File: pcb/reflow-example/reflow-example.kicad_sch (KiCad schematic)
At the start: 24 parts, among them U1 NE555D, U2 74LS47, U3 KCSA02-105, U4 74LS393, U5 74LS47, U6 KCSA02-105

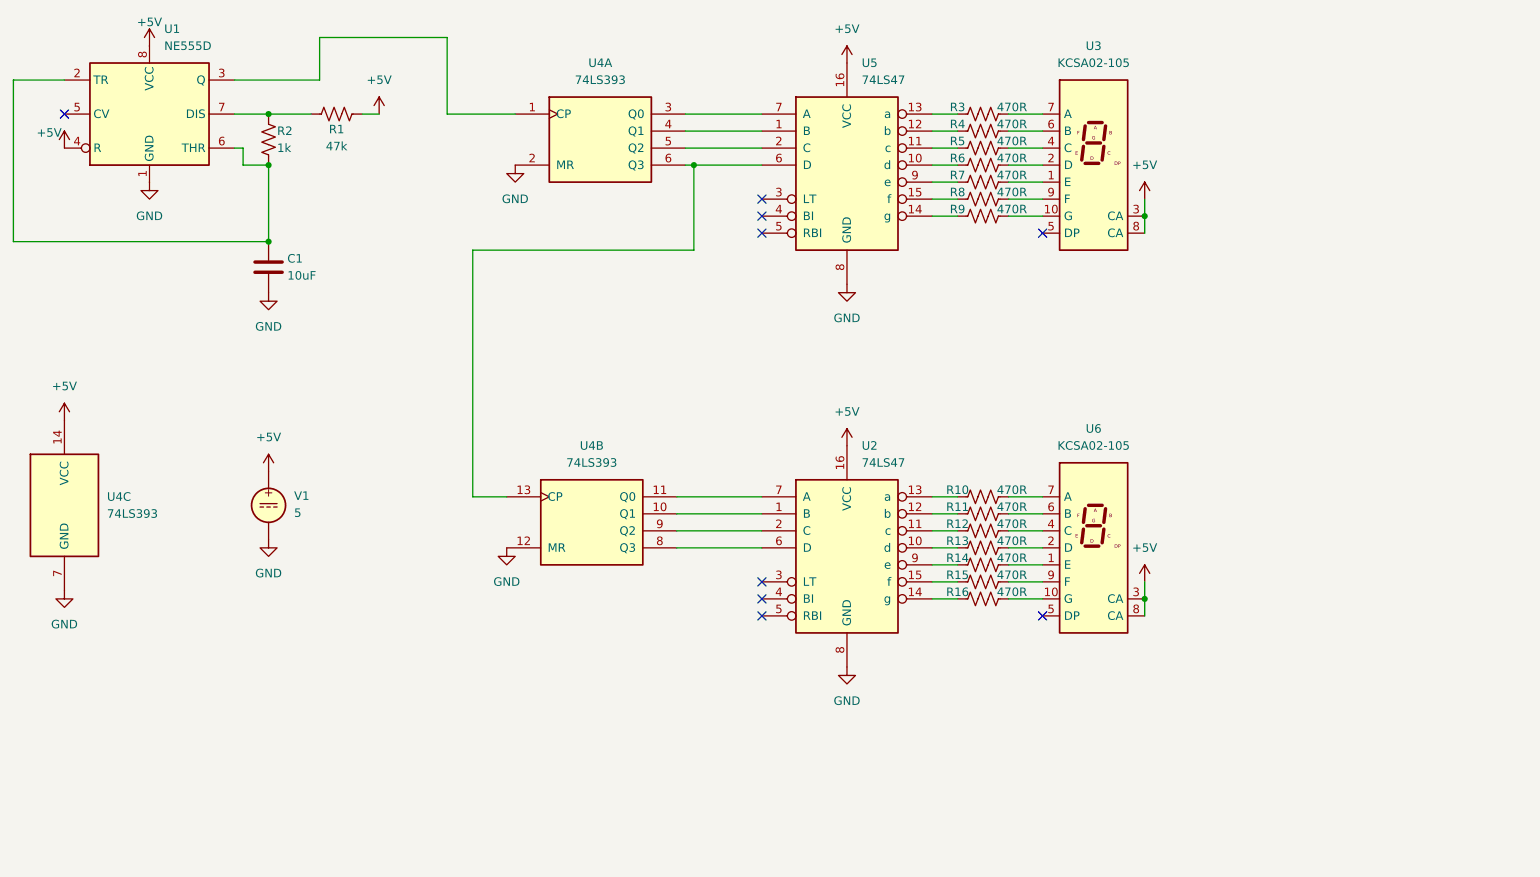
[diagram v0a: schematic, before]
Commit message: file a radar.
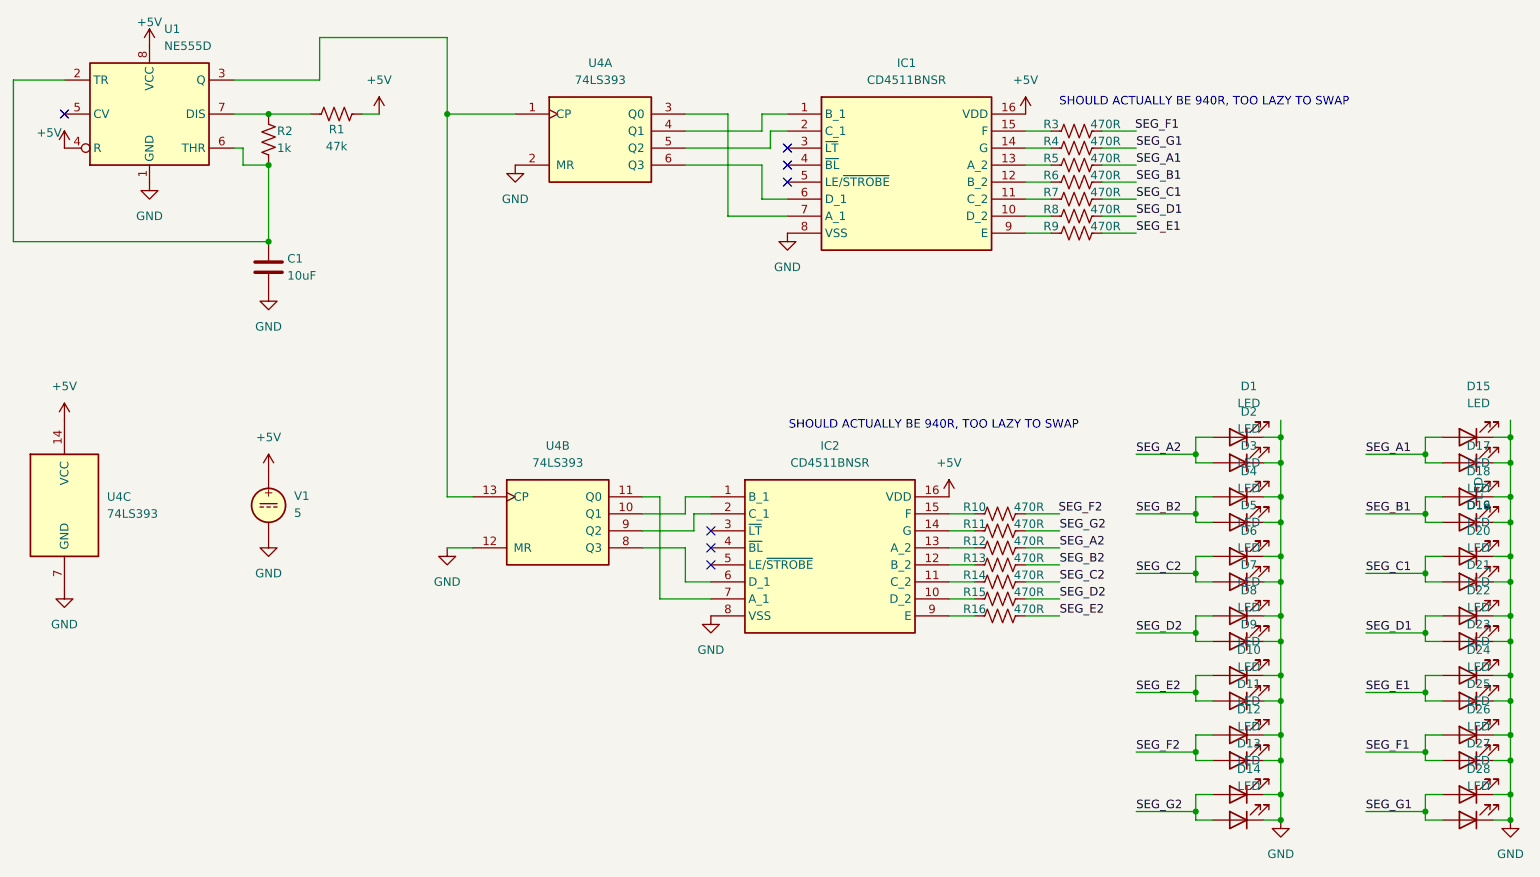
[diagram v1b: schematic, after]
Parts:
- removed U2, U5: 74LS47, symbol 74xx:74LS47
- removed U3, U6: KCSA02-105, Display_7Segment:HDSP-7401, symbol Display_Character:KCSA02-105
- added D1, D11, D13, D3, D5, D7, D9: LED, Diode_SMD:D_0402_1005Metric, symbol Device:LED
- added D10, D12, D14, D2, D4, D6, D8: LED, Diode_SMD:D_0603_1608Metric, symbol Device:LED
- added D15, D17, D19, D21, D23, D25, D27: LED, Diode_SMD:D_0805_2012Metric, symbol Device:LED
- added D16, D18, D20, D22, D24, D26, D28: LED, Diode_SMD:D_1206_3216Metric, symbol Device:LED
- added IC1, IC2: CD4511BNSR, KiCad:SOIC127P780X200-16N, symbol CD4511BNSR:CD4511BNSR
- C1, R1, R10, R11, R12, R13, R14, R15, R16, R2, R3, R4, R5, R6, R7, R8, R9: footprint (none) -> Capacitor_SMD:C_1206_3216Metric
- U4: footprint (none) -> Package_DIP:DIP-14_W7.62mm_SMDSocket_SmallPads
- V1: footprint (none) -> Connector_PinHeader_2.54mm:PinHeader_1x02_P2.54mm_Horizontal
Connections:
- net +5V: now also IC1.16 (VDD), IC2.16 (VDD)
- net GND: now also D1.1 (K), D10.1 (K), D11.1 (K), D12.1 (K), D13.1 (K), D14.1 (K), D15.1 (K), D16.1 (K), D17.1 (K), D18.1 (K), D19.1 (K), D2.1 (K), D20.1 (K), D21.1 (K), D22.1 (K), D23.1 (K), D24.1 (K), D25.1 (K), D26.1 (K), D27.1 (K), D28.1 (K), D3.1 (K), D4.1 (K), D5.1 (K), D6.1 (K), D7.1 (K), D8.1 (K), D9.1 (K), IC1.8 (VSS), IC2.8 (VSS)
- net at U4.10 (Q1): now also IC2.1 (B_1)
- net at U4.11 (Q0): now also IC2.7 (A_1)
- net at U4.13 (CP): now also U1.3 (Q), U4.1 (CP); no longer U4.6 (Q3)
- net at U4.8 (Q3): now also IC2.6 (D_1)
- net at U4.9 (Q2): now also IC2.2 (C_1)
- net at R10.1: now also IC2.15 (F)
- net SEG_F2: now reaches R10.2
- net SEG_F2: now also D11.2 (A), D12.2 (A)
- net at R13.1: now also IC2.12 (B_2)
- net at R12.1: now also IC2.13 (A_2)
- net at R11.1: now also IC2.14 (G)
- net at R16.1: now also IC2.9 (E)
- net at R15.1: now also IC2.10 (D_2)
- net at R14.1: now also IC2.11 (C_2)
- net SEG_A2: now reaches R12.2
- net SEG_A2: now also D1.2 (A), D2.2 (A)
- net at R7.1: now also IC1.11 (C_2)
- net SEG_C1: now reaches R7.2
- net SEG_C1: now also D19.2 (A), D20.2 (A)
- net at R9.1: now also IC1.9 (E)
- net SEG_E1: now reaches R9.2
- net SEG_E1: now also D23.2 (A), D24.2 (A)
- net SEG_E2: now reaches R16.2
- net SEG_E2: now also D10.2 (A), D9.2 (A)
- net SEG_B1: now reaches R6.2
- net SEG_B1: now also D17.2 (A), D18.2 (A)
- net SEG_A1: now reaches R5.2
- net SEG_A1: now also D15.2 (A), D16.2 (A)
- net SEG_G1: now reaches R4.2
- net SEG_G1: now also D27.2 (A), D28.2 (A)
- net SEG_F1: now reaches R3.2
- net SEG_F1: now also D25.2 (A), D26.2 (A)
- net SEG_D1: now reaches R8.2
- net SEG_D1: now also D21.2 (A), D22.2 (A)
- net SEG_C2: now reaches R14.2
- net SEG_C2: now also D5.2 (A), D6.2 (A)
- net SEG_B2: now reaches R13.2
- net SEG_B2: now also D3.2 (A), D4.2 (A)
- net SEG_G2: now reaches R11.2
- net SEG_G2: now also D13.2 (A), D14.2 (A)
- net SEG_D2: now reaches R15.2
- net SEG_D2: now also D7.2 (A), D8.2 (A)
- net at R6.1: now also IC1.12 (B_2)
- net at U4.3 (Q0): now also IC1.7 (A_1)
- net at U4.4 (Q1): now also IC1.1 (B_1)
- net at U4.5 (Q2): now also IC1.2 (C_1)
- net at R4.1: now also IC1.14 (G)
- net at R5.1: now also IC1.13 (A_2)
- net at R3.1: now also IC1.15 (F)
- net at R8.1: now also IC1.10 (D_2)
- new net: IC1.6 (D_1), U4.6 (Q3)
- no-connect marks 9 -> 7
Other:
- note added: "SHOULD ACTUALLY BE 940R, TOO LAZY TO SWAP"
- moved on the sheet: R3, R4, R5, R6, R7, R8, R9, U4B
